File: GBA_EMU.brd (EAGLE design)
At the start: 130.7 x 72.9 mm, 63 parts, among them J1 USB-MINIB-5PIN, Q1 MOSFET-PCHANNEL, SW1 LEFT, SW2 RIGHT, SW3 PWR_SWITCH, U2 FT230X, U4 LM4875, U5 V_REG_LDOSMD2, U7 AZV321, X2 HEADPHONE

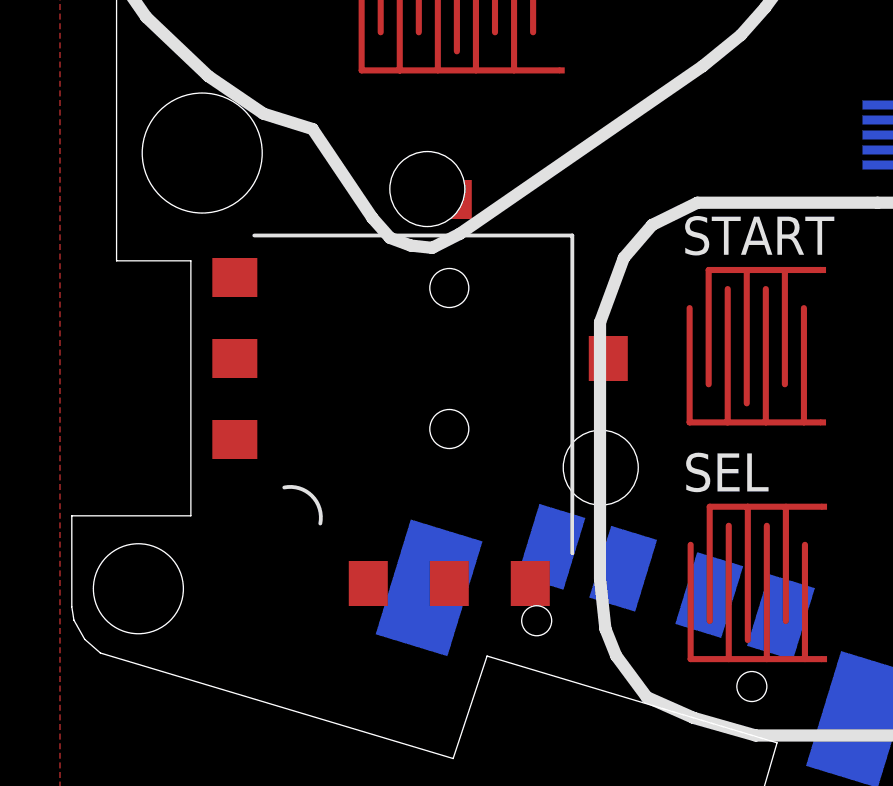
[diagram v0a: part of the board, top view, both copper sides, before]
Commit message: updated pdf render
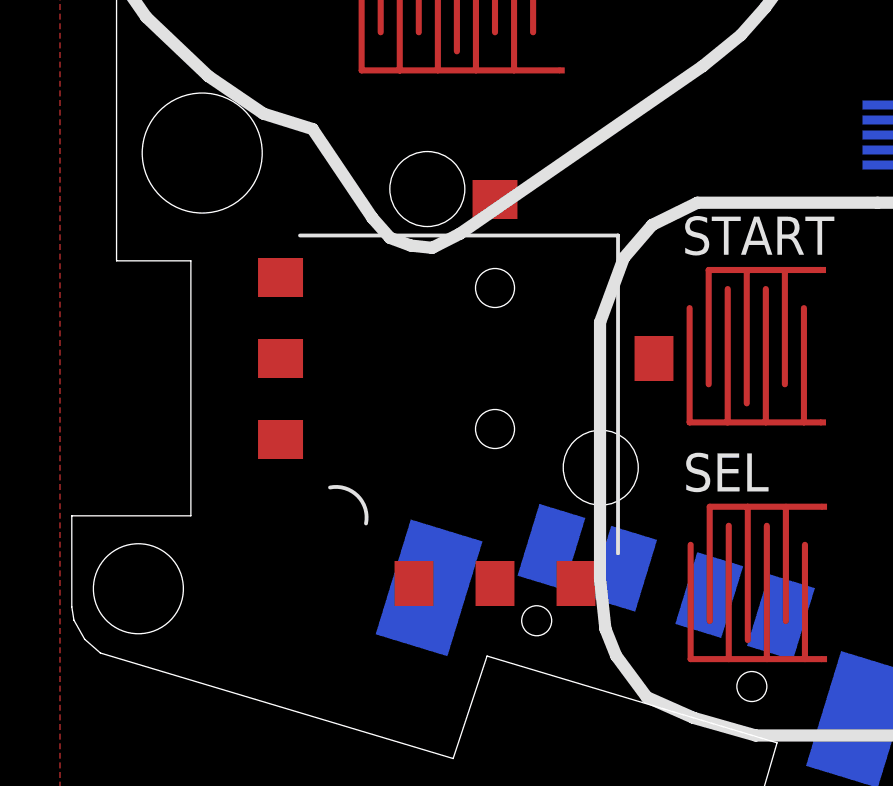
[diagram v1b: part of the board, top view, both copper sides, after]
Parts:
- moved U$4 1.52 mm to (29.0, 24.4)
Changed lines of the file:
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@@
 <element name="U$1" library="custom" package="S020-75MM" value="CBT3244AD" x="80.16" y="51.844" rot="R90"/>
 <element name="POT1" library="adafruit" package="THUMBWHEEL" value="THUMBPOT" x="91.2908" y="26.0612" rot="R195"/>
-<element name="U$4" library="custom" package="254SA103B50A" value="CTS254_JOYSTICKSM" x="27.432" y="24.384"/>
+<element name="U$4" library="custom" package="254SA103B50A" value="CTS254_JOYSTICKSM" x="28.956" y="24.384"/>
 <element name="SW4" library="adafruit" package="TACT_PANA-EVQ" value="" x="45.212" y="69.596"/>
 <element name="SW5" library="adafruit" package="TACT_PANA-EVQ" value="" x="121.412" y="69.596"/>
@@
 <wire x1="91.125" y1="73.025" x2="97.31125" y2="64.77" width="0" layer="19" extent="16-16"/>
 <wire x1="84.29875" y1="74.850625" x2="91.125" y2="73.025" width="0" layer="19" extent="16-16"/>
-<wire x1="33.932" y1="36.184" x2="26.782" y2="28.184" width="0" layer="19" extent="1-1"/>
-<wire x1="37.677790625" y1="45.56770625" x2="33.932" y2="36.184" width="0" layer="19" extent="1-1"/>
+<wire x1="35.456" y1="36.184" x2="28.306" y2="28.184" width="0" layer="19" extent="1-1"/>
+<wire x1="37.677790625" y1="45.56770625" x2="35.456" y2="36.184" width="0" layer="19" extent="1-1"/>
 <wire x1="29.69269375" y1="53.293165625" x2="37.677790625" y2="45.56770625" width="0" layer="19" extent="1-1"/>
 <wire x1="37.737625" y1="61.42204375" x2="45.69403125" y2="53.50889375" width="0" layer="19" extent="1-1"/>
 <wire x1="147" y1="28.575" x2="133.178471875" y2="27.330959375" width="0" layer="19" extent="16-16"/>
-<wire x1="125.524" y1="60.452" x2="36.632" y2="23.384" width="0" layer="19" extent="1-1"/>
+<wire x1="125.524" y1="60.452" x2="38.156" y2="23.384" width="0" layer="19" extent="1-1"/>
 <wire x1="139.24" y1="62.484" x2="125.524" y2="60.452" width="0" layer="19" extent="1-1"/>
 </signal>
@@
 <contactref element="U$4" pad="P$4"/>
 <contactref element="U$4" pad="P$5"/>
-<wire x1="31.232" y1="23.384" x2="26.782" y2="33.584" width="0" layer="19" extent="1-1"/>
-<wire x1="33.932" y1="23.384" x2="31.232" y2="23.384" width="0" layer="19" extent="1-1"/>
+<wire x1="32.756" y1="23.384" x2="28.306" y2="33.584" width="0" layer="19" extent="1-1"/>
+<wire x1="35.456" y1="23.384" x2="32.756" y2="23.384" width="0" layer="19" extent="1-1"/>
 </signal>
 <signal name="Z_BTN">
